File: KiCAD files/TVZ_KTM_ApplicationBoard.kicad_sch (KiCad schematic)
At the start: 64 parts, among them J1 Conn_02x19_Odd_Even, J2 Conn_02x19_Odd_Even, J3 Conn_02x19_Odd_Even, J4 Conn_02x19_Odd_Even, SW1 EG1271A, SW2 EG1271A, SW3 EG1271A, SW4 EG1271A, U1 LM75B, U2 MCP2551-I-P, U3 MCP2551-I-P

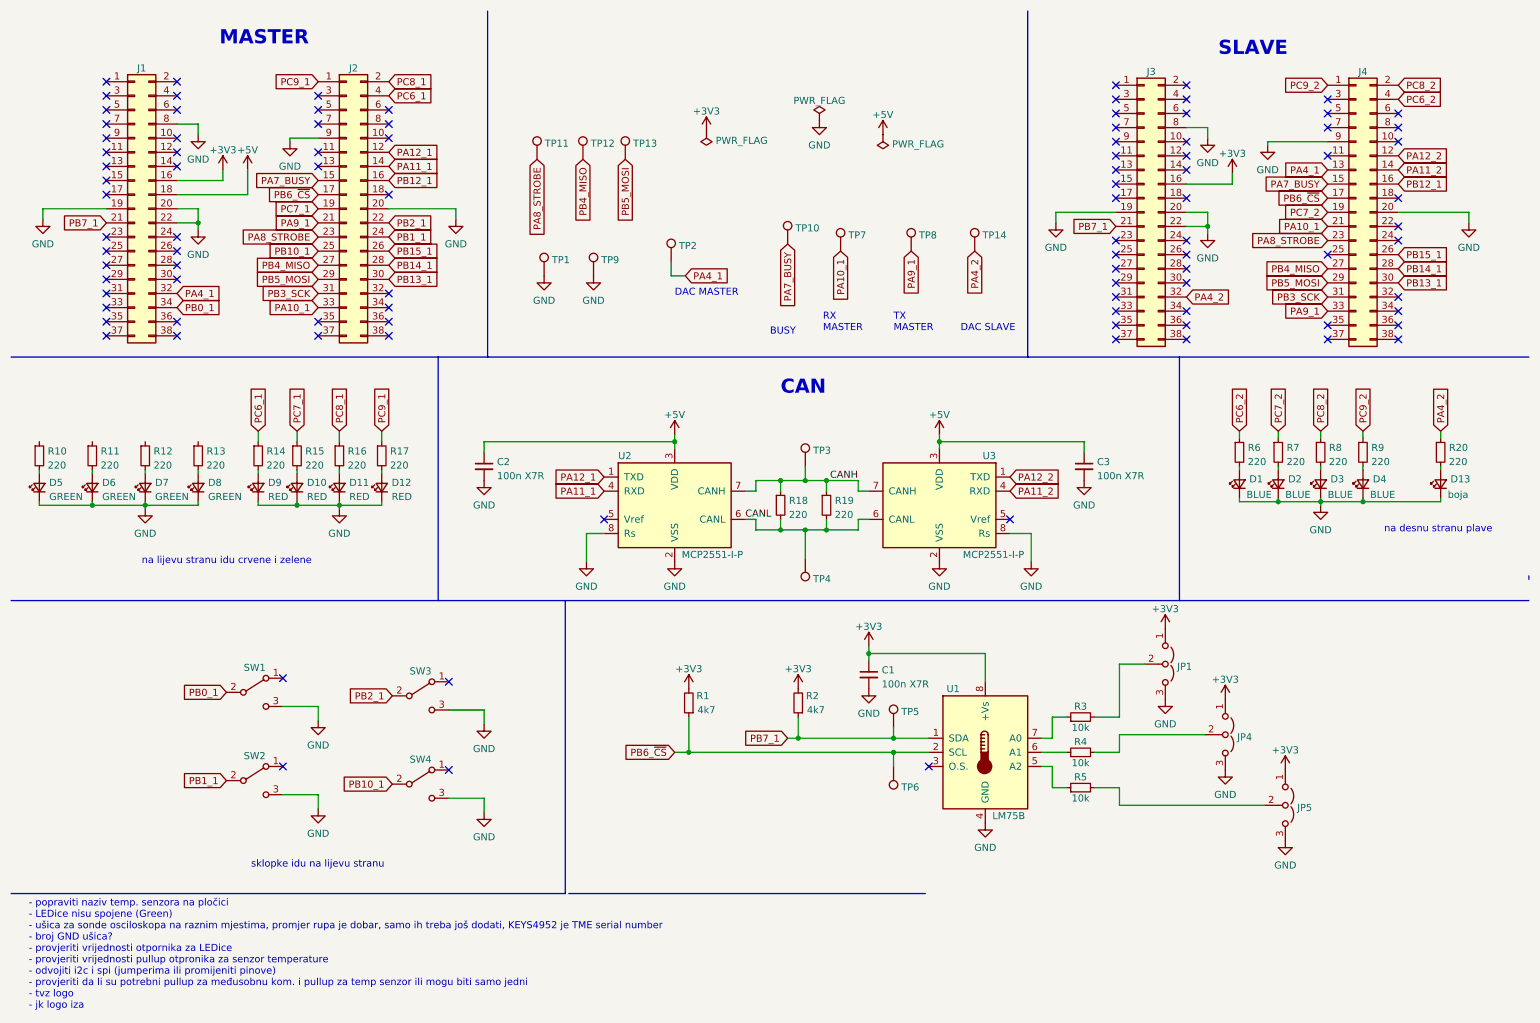
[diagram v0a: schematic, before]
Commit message: update
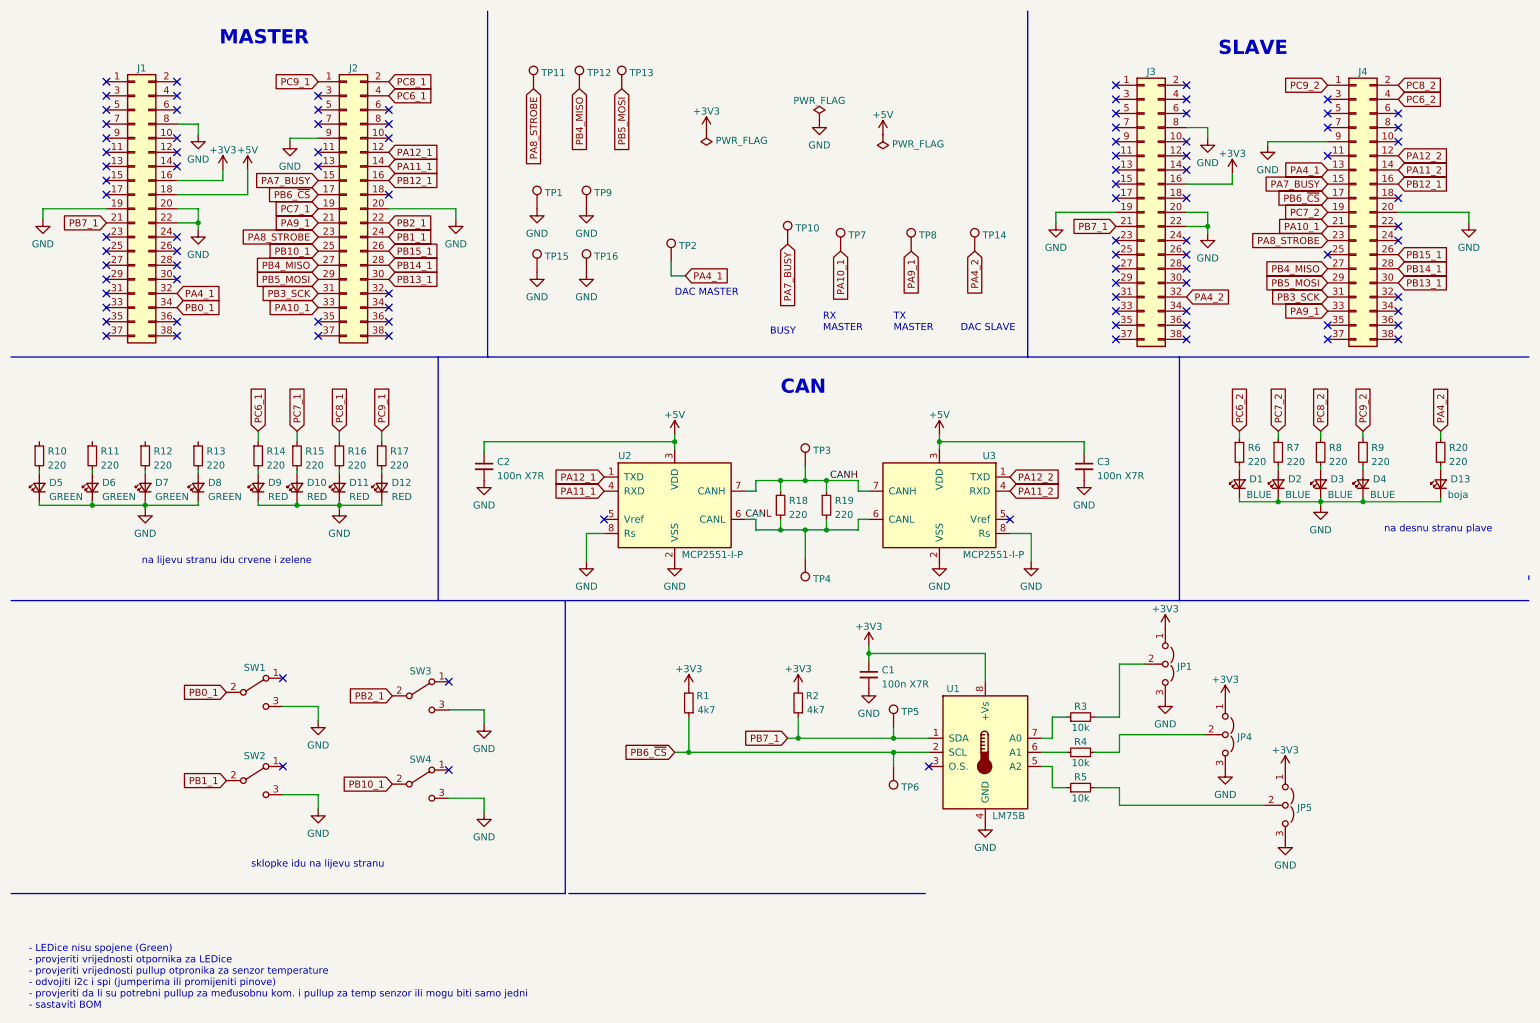
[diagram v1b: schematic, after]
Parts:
- added TP15, TP16: TestPoint, Footprint:KEYS4952, symbol Connector:TestPoint
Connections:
- net GND: now also TP15.1, TP16.1
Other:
- note added: "- LEDice nisu spojene (Green) - provjeriti vrijednosti otpornika za LEDice - provjeriti vrijednosti pullup otpronika za senzor temperature - odvojiti i2c i spi (jumperima ili promijeniti pinove) - provjeriti da li su potrebni pullup za međusobnu kom. i pullup za temp senzor ili mogu biti samo jedni - sastaviti BOM"
- note removed: "- popraviti naziv temp. senzora na pločici - LEDice nisu spojene (Green) - ušica za sonde osciloskopa na raznim mjestima, promjer rupa je dobar, samo ih treba još dodati, KEYS4952 je TME serial number - broj GND ušica? - provjeriti vrijednosti otpornika za LEDice - provjeriti vrijednosti pullup otpronika za senzor temperature - odvojiti i2c i spi (jumperima ili promijeniti pinove) - provjeriti da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"
- moved on the sheet: TP1, TP11, TP12, TP13, TP9
